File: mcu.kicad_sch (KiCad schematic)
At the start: 17 parts, among them U1 RP2040, U2 W25Q128JVS, Y1 Crystal_GND24

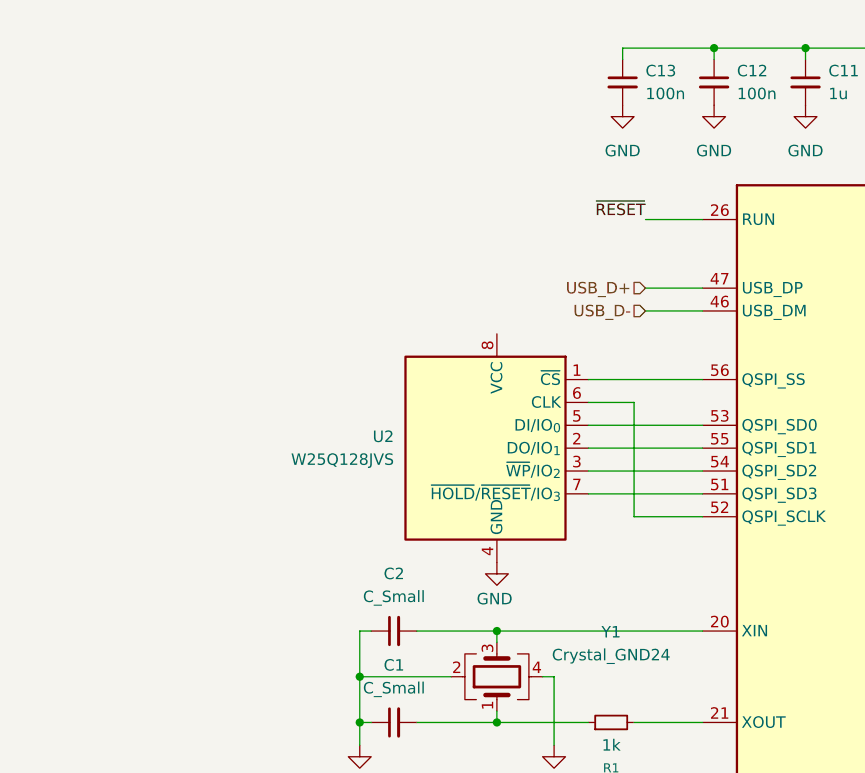
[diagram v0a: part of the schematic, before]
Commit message: add some TVS diodes
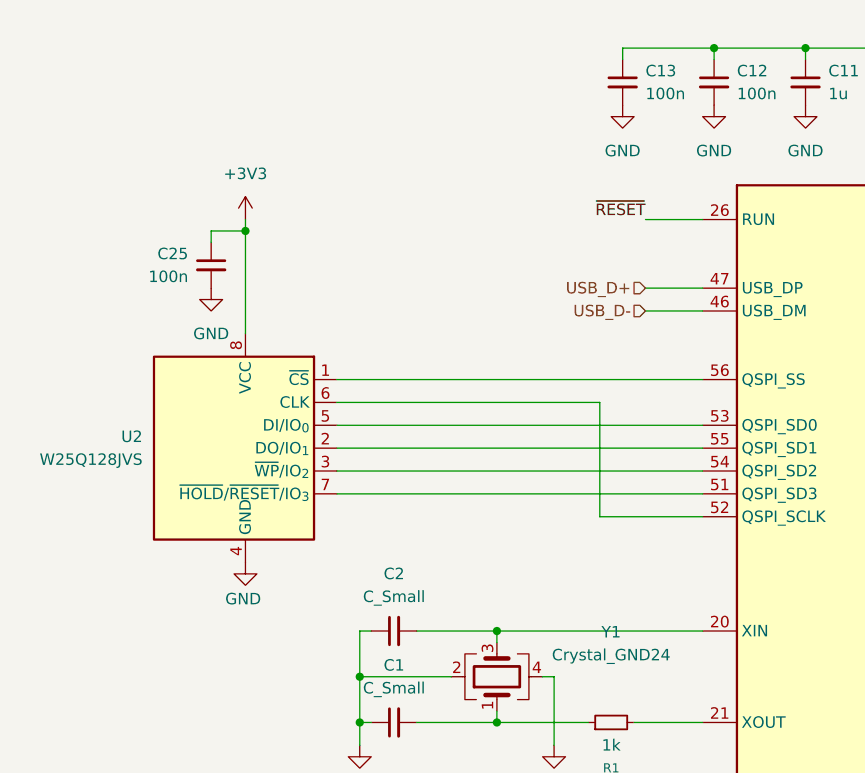
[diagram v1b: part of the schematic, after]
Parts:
- added C25: 100n, Capacitor_SMD:C_0402_1005Metric, symbol Device:C_Small
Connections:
- net +3V3: now also U2.8 (VCC), C25.1
- net GND: now also C25.2
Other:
- moved on the sheet: U2
